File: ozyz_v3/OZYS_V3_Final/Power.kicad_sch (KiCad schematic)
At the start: 31 parts, among them J1 Conn_01x02_Pin, Q1 AO3401A, Q3 AO3401A, U2 TPS63070RNMR, U3 AMS1117-3.3

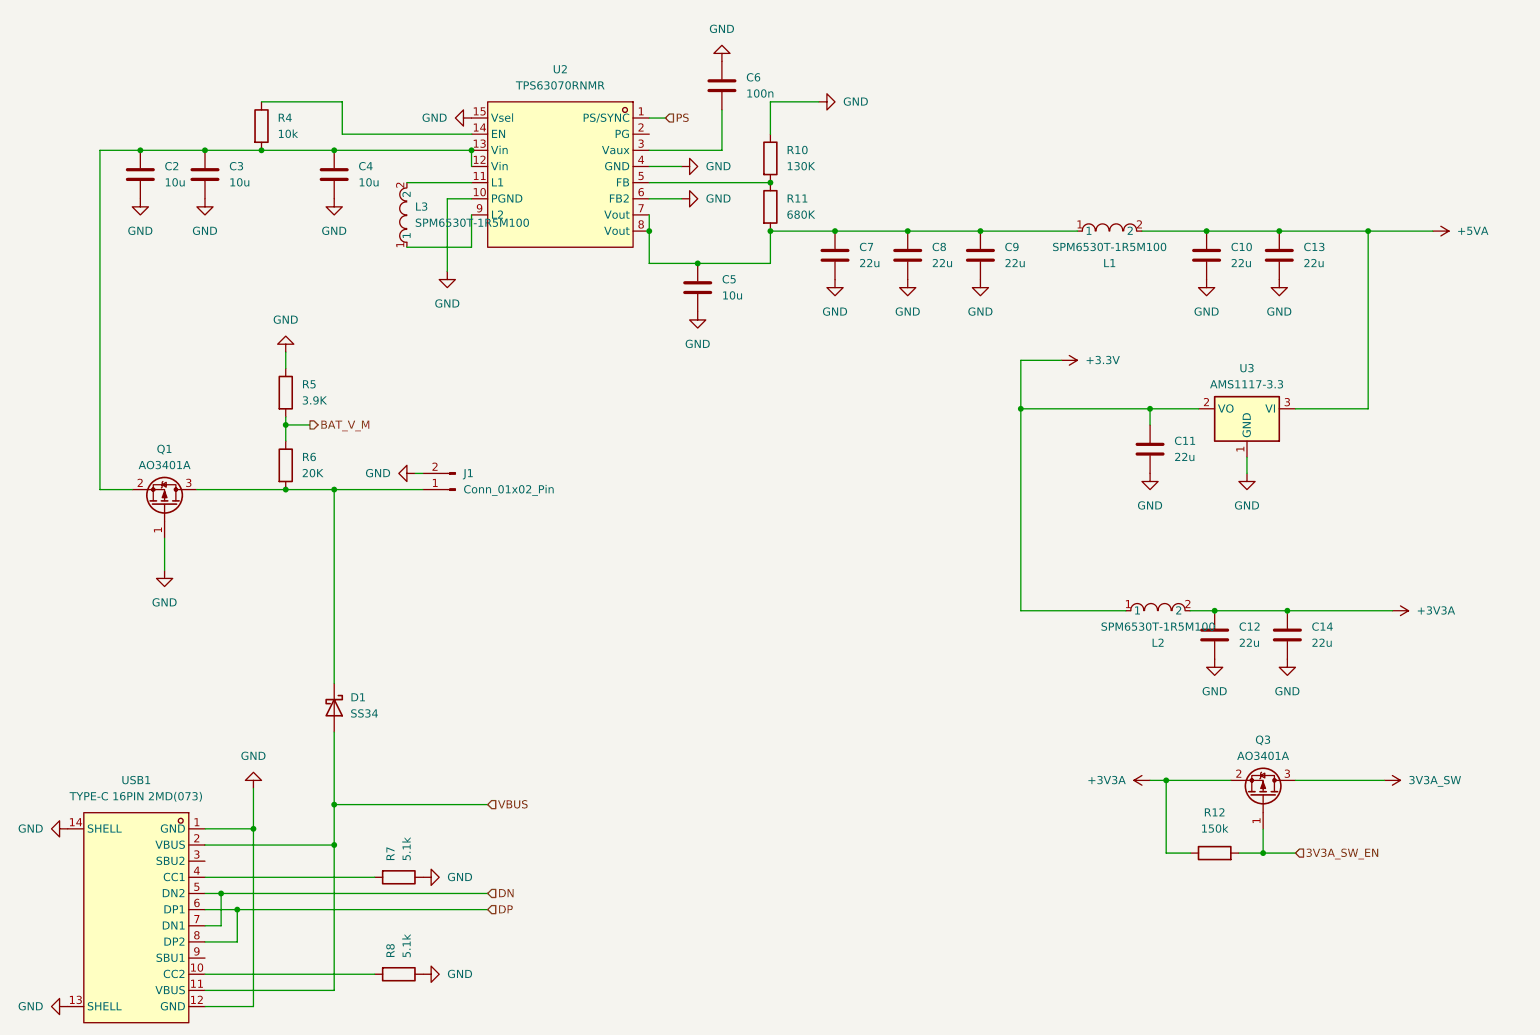
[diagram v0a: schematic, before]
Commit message: Yolo2
new Ozys
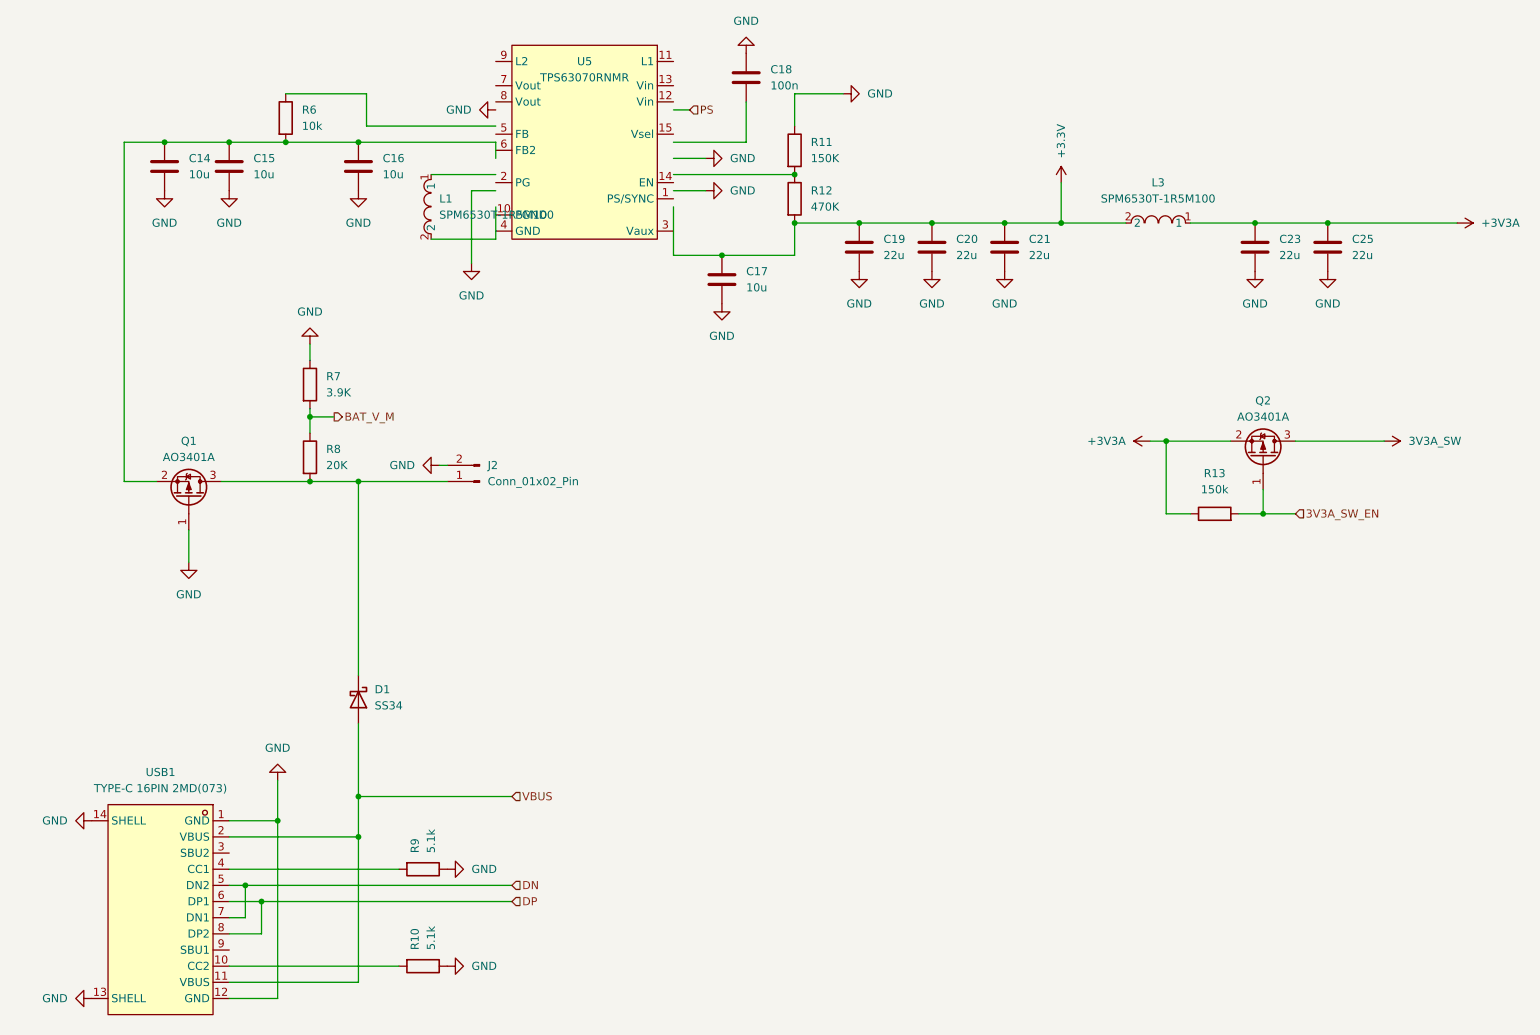
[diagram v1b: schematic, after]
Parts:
- removed C10, C11, C12, C13, C7, C8, C9: 22u, Capacitor_SMD:C_0603_1608Metric, symbol Device:C
- removed C2, C3, C4, C5: 10u, Capacitor_SMD:C_0603_1608Metric, symbol Device:C
- removed C6: 100n, Capacitor_SMD:C_0402_1005Metric, symbol Device:C
- removed J1: Conn_01x02_Pin, Rocketry_Manual:1054301102, symbol Connector:Conn_01x02_Pin
- removed L2: SPM6530T-1R5M100, Rocketry_Easyeda:IND-SMD_L7.1-W6.5-P5.60, symbol Rocketry_Easyeda:SPM6530T-1R5M100
- removed Q3: AO3401A, Package_TO_SOT_SMD:SOT-23, symbol Transistor_FET:AO3401A
- removed R4: 10k, Resistor_SMD:R_0402_1005Metric, symbol Device:R
- removed R5: 3.9K, Resistor_SMD:R_0603_1608Metric, symbol Device:R
- removed U2: TPS63070RNMR, Rocketry_Easyeda:VQFN-HR-15_L3.0-W2.5-P0.50-BL_TPS63070RNMR, symbol Rocketry_Easyeda:TPS63070RNMR
- removed U3: AMS1117-3.3, Package_TO_SOT_SMD:SOT-223-3_TabPin2, symbol Regulator_Linear:AMS1117-3.3
- added C15, C16, C17: 10u, Capacitor_SMD:C_0603_1608Metric, symbol Device:C
- added C18: 100n, Capacitor_SMD:C_0402_1005Metric, symbol Device:C
- added C19, C20, C21, C23, C25: 22u, Capacitor_SMD:C_0603_1608Metric, symbol Device:C
- added J2: Conn_01x02_Pin, Rocketry_Manual:1054301102, symbol Connector:Conn_01x02_Pin
- added Q2: AO3401A, Package_TO_SOT_SMD:SOT-23, symbol Transistor_FET:AO3401A
- added R13: 150k, Resistor_SMD:R_0603_1608Metric, symbol Device:R
- added R9: 5.1k, Resistor_SMD:R_0402_1005Metric, symbol Device:R
- added U5: TPS63070RNMR, Rocketry_Easyeda:VQFN-HR-15_L3.0-W2.5-P0.50-BL_TPS63070RNMR, symbol Rocketry_Easyeda:TPS63070RNMR
- C14: value 22u -> 10u
- R10: value 130K -> 5.1k; footprint Resistor_SMD:R_0603_1608Metric -> Resistor_SMD:R_0402_1005Metric
- R11: value 680K -> 150K; footprint Resistor_SMD:R_0402_1005Metric -> Resistor_SMD:R_0603_1608Metric
- R12: value 150k -> 470K; footprint Resistor_SMD:R_0603_1608Metric -> Resistor_SMD:R_0402_1005Metric
- R6: value 20K -> 10k
- R7: value 5.1k -> 3.9K; footprint Resistor_SMD:R_0402_1005Metric -> Resistor_SMD:R_0603_1608Metric
- R8: value 5.1k -> 20K
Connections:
- net +3.3V: now also L3.2, R12.2, C17.2, C19.2, C20.2, C21.2
- net +3V3A: now also L3.1, C23.2, C25.2, Q2.2 (S), R13.1; no longer C14.2, R12.1
- net 3V3A_SW: now also Q2.3 (D)
- net 3V3A_SW_EN: now also Q2.1 (G), R13.2; no longer R12.2
- net BAT_V_M: now also R7.2, R8.1; no longer R6.1
- net GND: now also R11.1, C15.1, C16.1, C17.1, C18.2, C19.1, C20.1, C21.1, C23.1, C25.1, J2.2 (Pin_2), R9.1; no longer R8.1
- net at Q1.2 (S): now also C14.2, R6.2, C15.2, C16.2
- net at D1.1 (K), Q1.3 (D): now also R8.2, J2.1 (Pin_1); no longer R6.2
- net at R10.2: now also USB1.10 (CC2); no longer R11.1
- net at R11.2: now also R12.1; no longer L1.1
- net at USB1.4 (CC1): now also R9.2; no longer R7.2
- net +5VA: no longer names the net of L1.2
